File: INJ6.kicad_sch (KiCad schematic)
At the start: 12 parts, among them Q13 ZXMS6005SGTA, Q14 ZXMS6005SGTA, Q15 ZXMS6005SGTA, Q16 ZXMS6005SGTA, Q17 ZXMS6005SGTA, Q18 ZXMS6005SGTA

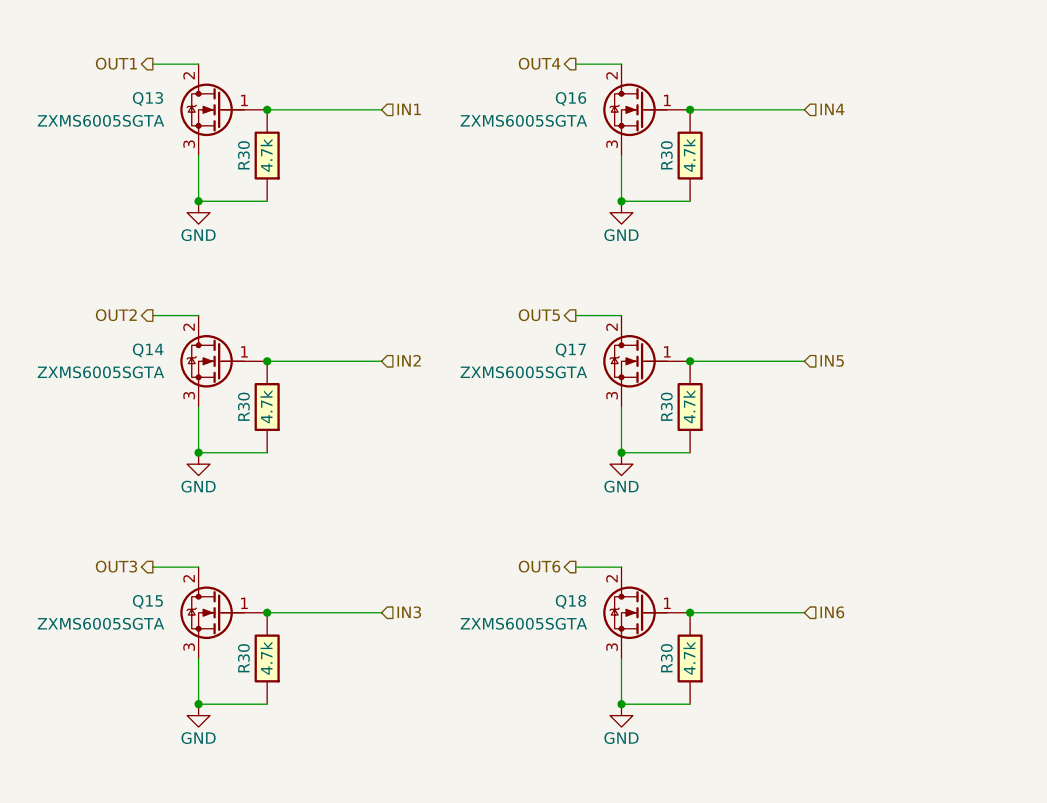
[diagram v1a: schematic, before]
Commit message: Upd SCH, PCB
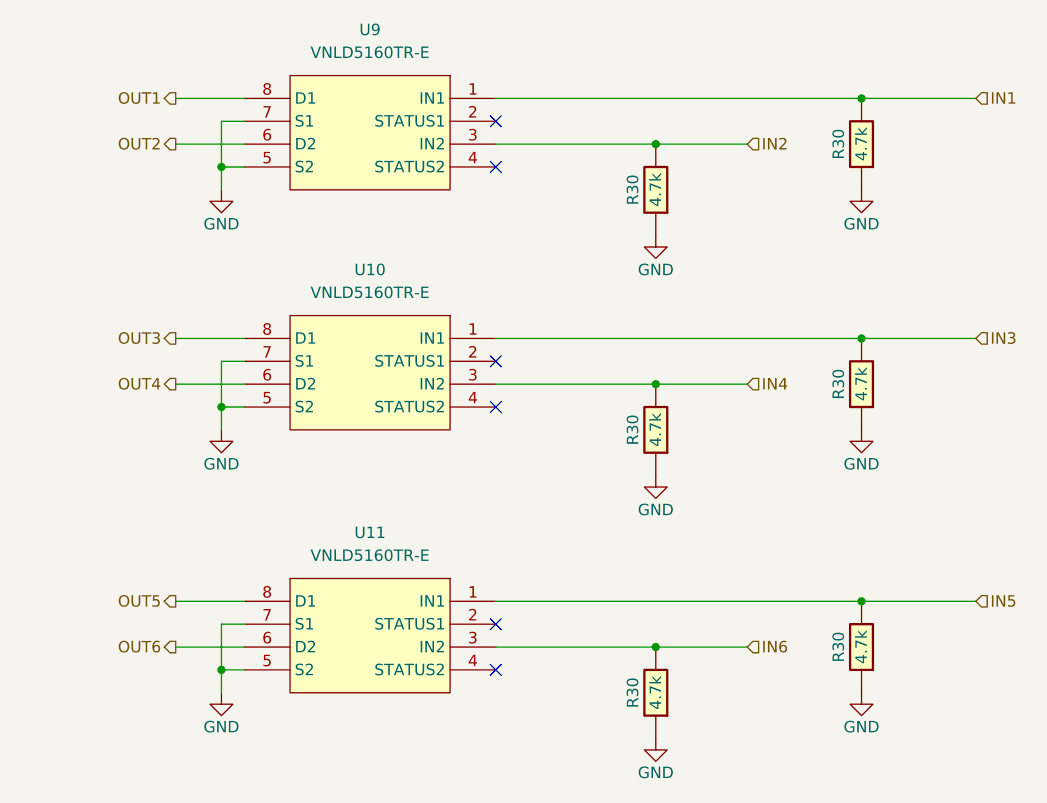
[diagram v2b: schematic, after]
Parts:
- removed Q13, Q14, Q15, Q16, Q17, Q18: ZXMS6005SGTA, Package_TO_SOT_SMD:SOT-223, symbol Transistor_FET:BSP129
- added U10, U11, U9: VNLD5160TR-E, Package_SO:SOIC-8_3.9x4.9mm_P1.27mm, symbol chips:VNLD5160
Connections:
- net GND: now also U10.5 (S2), U10.7 (S1), U11.5 (S2), U11.7 (S1), U9.5 (S2), U9.7 (S1)
- net IN1: now also U9.1 (IN1)
- net IN2: now also U9.3 (IN2)
- net IN3: now also U10.1 (IN1)
- net IN4: now also U10.3 (IN2)
- net IN5: now also U11.1 (IN1)
- net IN6: now also U11.3 (IN2)
- net OUT1: now also U9.8 (D1)
- net OUT2: now also U9.6 (D2)
- net OUT3: now also U10.8 (D1)
- net OUT4: now also U10.6 (D2)
- net OUT5: now also U11.8 (D1)
- net OUT6: now also U11.6 (D2)
- no-connect marks 0 -> 6
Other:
- moved on the sheet: R30
